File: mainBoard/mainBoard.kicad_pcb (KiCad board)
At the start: 2 copper layers, 35 x 52.1 mm, 29 parts, among them J1 Conn_01x01, J2 Conn_01x06_Male, J3 Conn_01x06_Male, J4 Conn_01x03_Male, Q1 SS8050-G, Q2 SS8050-G, SW1 SW_Push, SW2 SW_Push, U1 AMS1117-3.3, U2 ESP32-WROOM-E

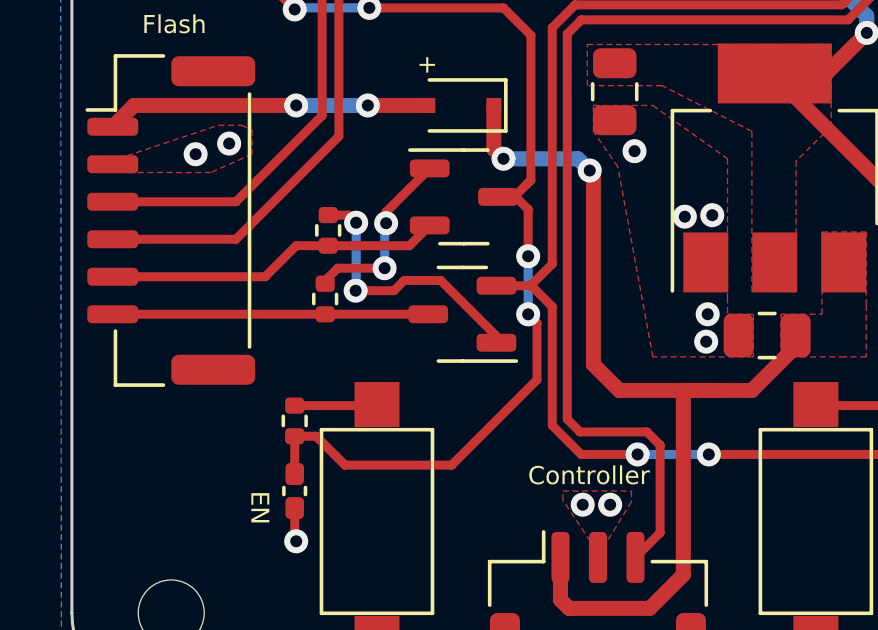
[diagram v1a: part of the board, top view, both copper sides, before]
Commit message: connector and emitter switched
maybe a problem maybe not
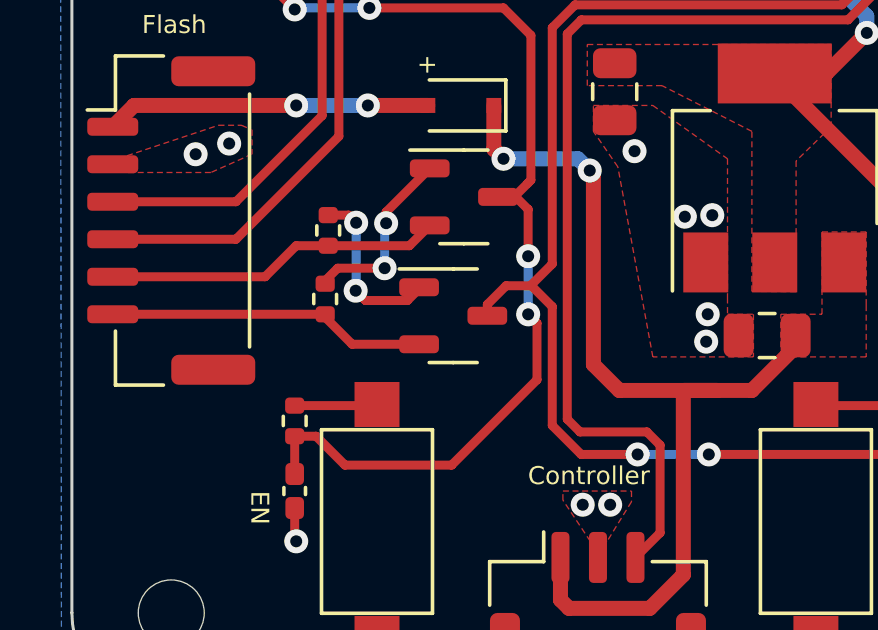
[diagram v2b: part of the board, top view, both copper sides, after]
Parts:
- SW1, SW2: value SW_Push -> C520860
- moved Q2 0.31 mm to (92.7, 87.6), turned to 0 degrees
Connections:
- Q2 pad 2: /Boot -> /DTR
- Q2 pad 3: /DTR -> /Boot
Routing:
- net Net-(Q2-Pad1): track 9.13 -> 5.77 mm
- net /Boot: track 41.7 -> 42.6 mm
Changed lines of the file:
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@@
     (property "Sheetfile" "mainBoard.kicad_sch")
     (property "Sheetname" "")
-    (attr exclude_from_pos_files exclude_from_bom)
+    (attr exclude_from_pos_files)
     (fp_text reference "J1" (at 0 -2.286) (layer "F.Fab")
       (effects (font (size 1 1) (thickness 0.15)))
@@
     (property "Sheetfile" "mainBoard.kicad_sch")
     (property "Sheetname" "")
-    (attr exclude_from_pos_files exclude_from_bom)
+    (attr exclude_from_pos_files)
     (fp_text reference "H2" (at 0 -3.2) (layer "F.Fab")
       (effects (font (size 1 1) (thickness 0.15)))
@@
     (property "Sheetfile" "mainBoard.kicad_sch")
     (property "Sheetname" "")
-    (attr exclude_from_pos_files exclude_from_bom)
+    (attr exclude_from_pos_files)
     (fp_text reference "H1" (at 0 -3.2) (layer "F.Fab")
       (effects (font (size 1 1) (thickness 0.15)))
@@
     (property "Sheetfile" "mainBoard.kicad_sch")
     (property "Sheetname" "")
-    (attr exclude_from_pos_files exclude_from_bom)
+    (attr exclude_from_pos_files)
     (fp_text reference "H4" (at 0 -3.2) (layer "F.Fab")
       (effects (font (size 1 1) (thickness 0.15)))
@@
       (effects (font (size 1 1) (thickness 0.15)))
     )
-    (fp_text value "SW_Push" (at 0 3 90) (layer "F.Fab")
+    (fp_text value "C520860" (at 0 3 90) (layer "F.Fab")
       (effects (font (size 1 1) (thickness 0.15)))
     )
@@
   )
   (footprint "Package_TO_SOT_SMD:SOT-23-3" (layer "F.Cu")
-    (at 93.0148 87.5792 180)
+    (at 92.71 87.63)
     (descr "SOT, 3 Pin (https://www.jedec.org/sites/default/files/docs/Mo-178D.PDF inferred 3-pin variant), generated with kicad-footprint-generator ipc_gullwing_generator.py")
     (tags "SOT TO_SOT_SMD")
@@
     (fp_line (start -0.8 1.45) (end -0.8 -1.05) (layer "F.Fab") (width 0.1))
     (fp_line (start 0.8 -1.45) (end 0.8 1.45) (layer "F.Fab") (width 0.1))
-    (pad "1" smd roundrect locked (at -1.1375 -0.95 180) (size 1.325 0.6) (layers "F.Cu" "F.Paste" "F.Mask") (roundrect_rratio 0.25)
+    (pad "1" smd roundrect locked (at -1.1375 -0.95) (size 1.325 0.6) (layers "F.Cu" "F.Paste" "F.Mask") (roundrect_rratio 0.25)
       (net 18 "Net-(Q2-Pad1)") (pinfunction "B") (pintype "input"))
-    (pad "2" smd roundrect locked (at -1.1375 0.95 180) (size 1.325 0.6) (layers "F.Cu" "F.Paste" "F.Mask") (roundrect_rratio 0.25)
-      (net 5 "/Boot") (pinfunction "E") (pintype "passive"))
-    (pad "3" smd roundrect locked (at 1.1375 0 180) (size 1.325 0.6) (layers "F.Cu" "F.Paste" "F.Mask") (roundrect_rratio 0.25)
-      (net 15 "/DTR") (pinfunction "C") (pintype "passive"))
+    (pad "2" smd roundrect locked (at -1.1375 0.95) (size 1.325 0.6) (layers "F.Cu" "F.Paste" "F.Mask") (roundrect_rratio 0.25)
+      (net 15 "/DTR") (pinfunction "E") (pintype "passive"))
+    (pad "3" smd roundrect locked (at 1.1375 0) (size 1.325 0.6) (layers "F.Cu" "F.Paste" "F.Mask") (roundrect_rratio 0.25)
+      (net 5 "/Boot") (pinfunction "C") (pintype "passive"))
     (model "${KICAD6_3DMODEL_DIR}/Package_TO_SOT_SMD.3dshapes/SOT-23-3.wrl"
       (offset (xyz 0 0 0))
@@
       (effects (font (size 1 1) (thickness 0.15)))
     )
-    (fp_text value "SW_Push" (at 0 3 90) (layer "F.Fab")
+    (fp_text value "C520860" (at 0 3 90) (layer "F.Fab")
       (effects (font (size 1 1) (thickness 0.15)))
     )
@@
     (property "Sheetfile" "mainBoard.kicad_sch")
     (property "Sheetname" "")
-    (attr exclude_from_pos_files exclude_from_bom)
+    (attr exclude_from_pos_files)
     (fp_text reference "H3" (at 0 -3.2) (layer "F.Fab")
       (effects (font (size 1 1) (thickness 0.15)))
@@
   (segment (start 107.4928 92.9553) (end 107.4928 92.2528) (width 0.3) (layer "F.Cu") (net 5))
   (segment (start 95.316 86.5988) (end 96.012 85.9028) (width 0.3) (layer "F.Cu") (net 5))
+  (segment (start 93.8475 87.63) (end 93.8475 87.2545) (width 0.3) (layer "F.Cu") (net 5))
   (segment (start 105.664 77.2668) (end 106.286 76.6448) (width 0.3) (layer "F.Cu") (net 5))
   (segment (start 107.4928 92.2528) (end 101.2303 92.2528) (width 0.3) (layer "F.Cu") (net 5))
@@
   (segment (start 96.012 78.0288) (end 96.774 77.2668) (width 0.3) (layer "F.Cu") (net 5))
   (segment (start 106.286 76.6448) (end 106.286 73.992) (width 0.3) (layer "F.Cu") (net 5))
+  (segment (start 94.4728 86.6292) (end 95.316 86.6292) (width 0.3) (layer "F.Cu") (net 5))
   (segment (start 96.9772 92.2528) (end 96.012 91.2876) (width 0.3) (layer "F.Cu") (net 5))
-  (segment (start 95.316 86.6292) (end 94.1523 86.6292) (width 0.3) (layer "F.Cu") (net 5))
+  (segment (start 93.8475 87.2545) (end 94.4728 86.6292) (width 0.3) (layer "F.Cu") (net 5))
   (segment (start 96.012 91.2876) (end 96.012 87.3252) (width 0.3) (layer "F.Cu") (net 5))
   (segment (start 95.316 86.6292) (end 95.316 86.5988) (width 0.3) (layer "F.Cu") (net 5))
@@
   (segment (start 88.5444 85.2952) (end 91.2505 85.2952) (width 0.3) (layer "F.Cu") (net 14))
   (segment (start 87.4756 85.2952) (end 86.4408 86.33) (width 0.3) (layer "F.Cu") (net 14))
-  (segment (start 88.4428 87.5812) (end 88.4416 87.58) (width 0.3) (layer "F.Cu") (net 15))
-  (segment (start 88.4428 87.5812) (end 88.4448 87.5792) (width 0.3) (layer "F.Cu") (net 15))
   (segment (start 88.4416 87.58) (end 81.362 87.58) (width 0.3) (layer "F.Cu") (net 15))
-  (segment (start 88.4448 87.5792) (end 91.8773 87.5792) (width 0.3) (layer "F.Cu") (net 15))
+  (segment (start 89.342 88.58) (end 88.4428 87.6808) (width 0.3) (layer "F.Cu") (net 15))
+  (segment (start 88.4428 87.6808) (end 88.4428 87.5812) (width 0.3) (layer "F.Cu") (net 15))
+  (segment (start 89.342 88.58) (end 91.5725 88.58) (width 0.3) (layer "F.Cu") (net 15))
   (segment (start 99.6068 91.942139) (end 99.167461 91.5028) (width 0.3) (layer "F.Cu") (net 16))
   (segment (start 107.3676 71.452) (end 106.286 71.452) (width 0.3) (layer "F.Cu") (net 16))
@@
   (segment (start 90.4748 84.5457) (end 90.424 84.5965) (width 0.3) (layer "B.Cu") (net 17))
   (segment (start 90.424 84.5965) (end 90.424 86.0447) (width 0.3) (layer "B.Cu") (net 17))
-  (segment (start 91.076081 86.45328) (end 92.29528 86.45328) (width 0.3) (layer "F.Cu") (net 18))
+  (segment (start 89.7866 87.122) (end 91.186 87.122) (width 0.3) (layer "F.Cu") (net 18))
   (segment (start 89.221717 84.2752) (end 89.475438 84.528921) (width 0.3) (layer "F.Cu") (net 18))
-  (segment (start 90.734661 86.7947) (end 91.076081 86.45328) (width 0.3) (layer "F.Cu") (net 18))
-  (segment (start 92.29528 86.45328) (end 94.1523 88.3103) (width 0.3) (layer "F.Cu") (net 18))
   (segment (start 88.5444 84.2752) (end 89.221717 84.2752) (width 0.3) (layer "F.Cu") (net 18))
-  (segment (start 89.4588 86.7942) (end 89.4593 86.7947) (width 0.3) (layer "F.Cu") (net 18))
-  (segment (start 89.4593 86.7947) (end 90.734661 86.7947) (width 0.3) (layer "F.Cu") (net 18))
-  (segment (start 94.1523 88.3103) (end 94.1523 88.5292) (width 0.3) (layer "F.Cu") (net 18))
+  (segment (start 91.186 87.122) (end 91.5725 86.7355) (width 0.3) (layer "F.Cu") (net 18))
+  (segment (start 91.5725 86.7355) (end 91.5725 86.68) (width 0.3) (layer "F.Cu") (net 18))
+  (segment (start 89.4588 86.7942) (end 89.7866 87.122) (width 0.3) (layer "F.Cu") (net 18))
   (via (at 89.475438 84.528921) (size 0.8) (drill 0.4) (layers "F.Cu" "B.Cu") (net 18))
   (via (at 89.4588 86.7942) (size 0.8) (drill 0.4) (layers "F.Cu" "B.Cu") (net 18))
